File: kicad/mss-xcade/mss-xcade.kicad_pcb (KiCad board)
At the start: 2 copper layers, 82.6 x 76.2 mm, 93 parts, among them J1 Screw_Terminal_01x02, J10 Screw_Terminal_01x02, J2 SM04B-SRSS, J3 SM04B-SRSS, J4 SM04B-SRSS, J5 8P8C, J6 8P8C, J7 AVR-ISP, J8 Screw_Terminal_01x02, J9 Screw_Terminal_01x02, U1 AP7381-50Y, U2 ATtiny861A-S, U3 74HC4049, U4 AP3012

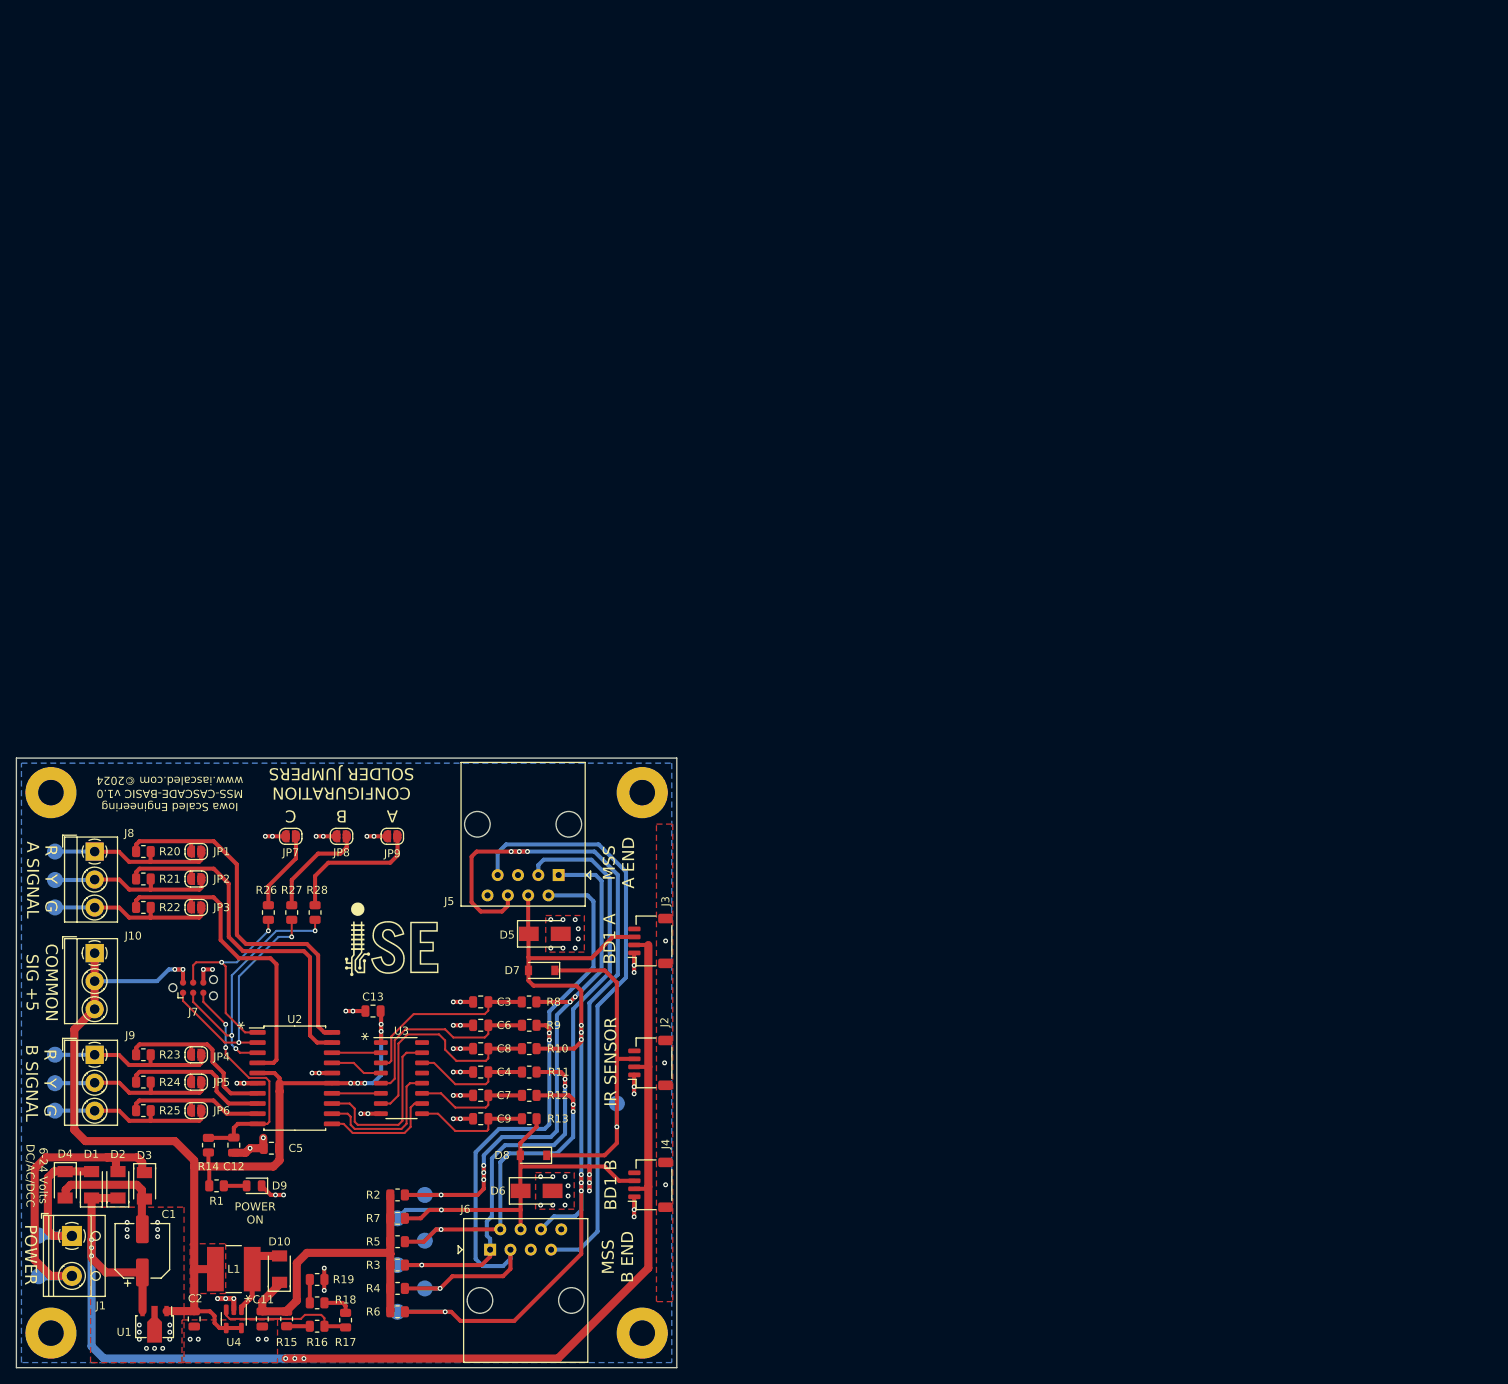
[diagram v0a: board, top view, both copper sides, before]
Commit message: First cut of xcade PCB
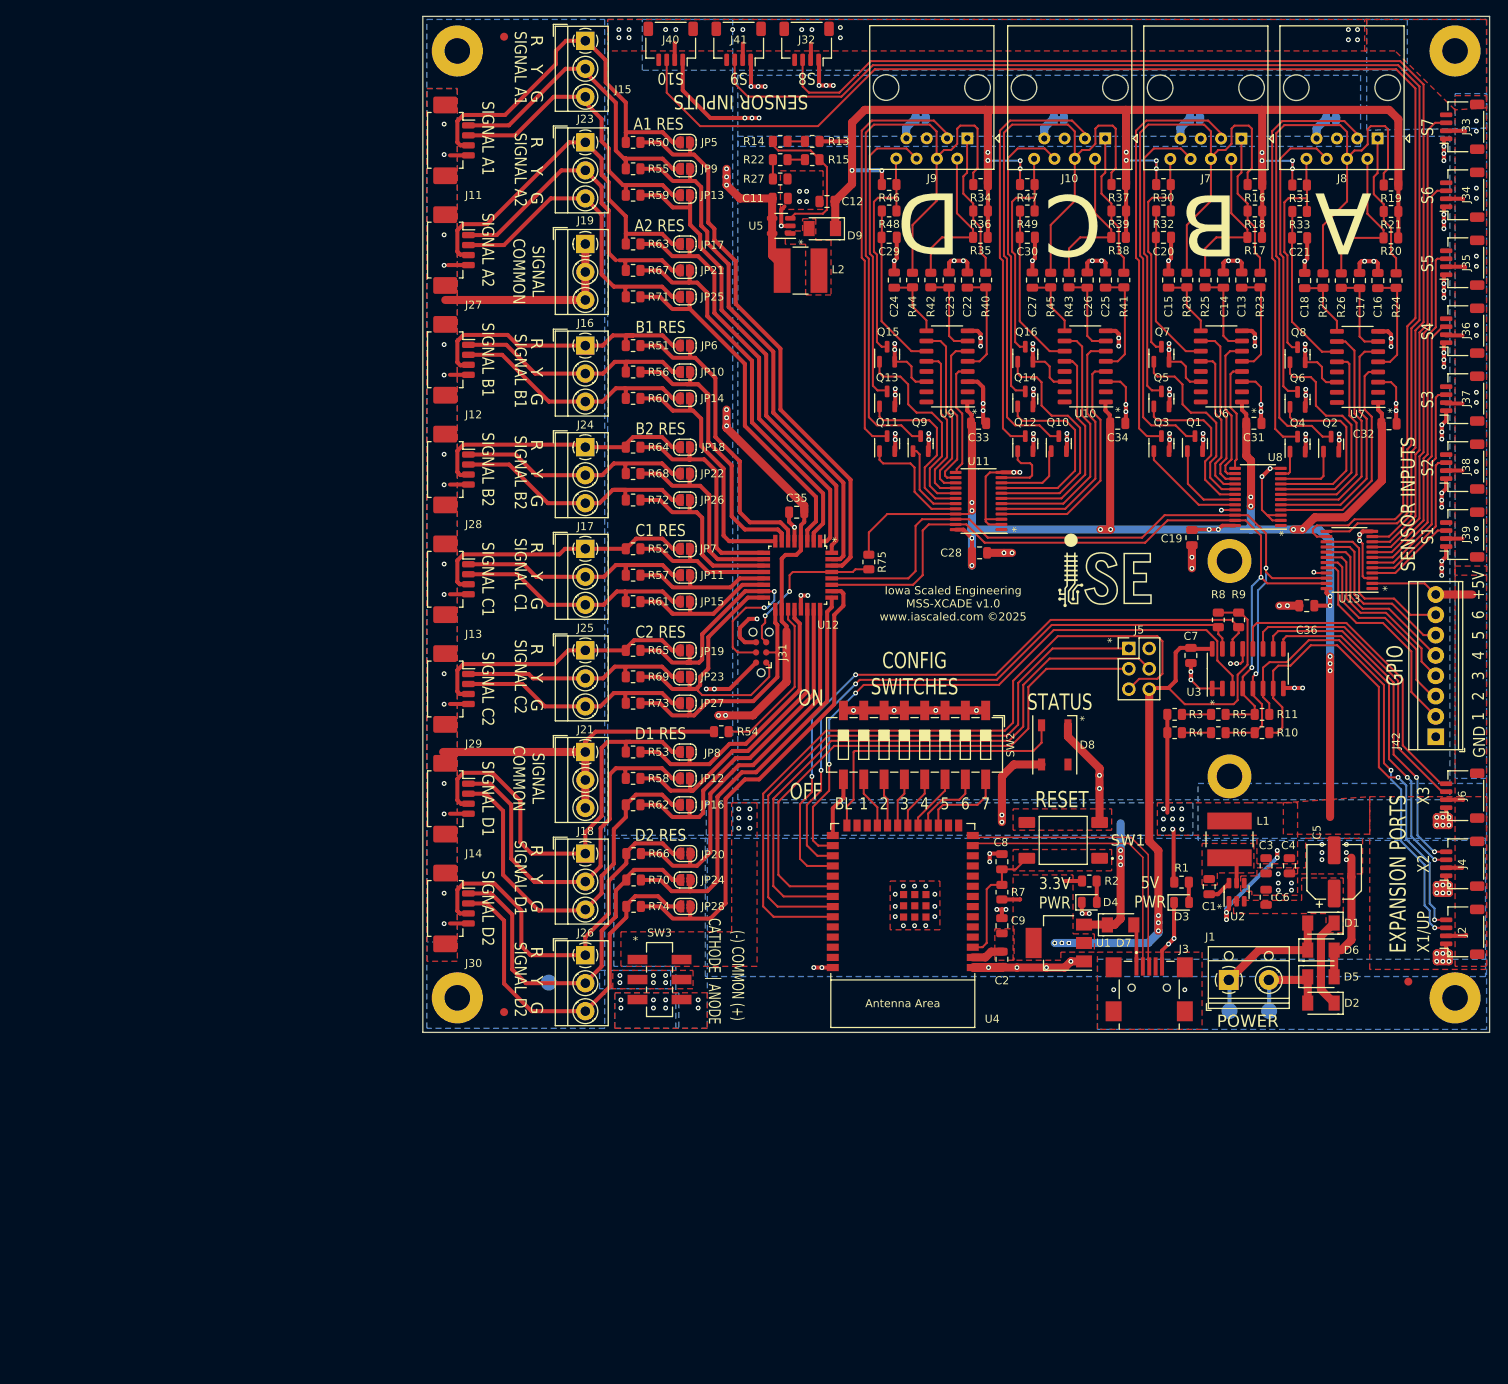
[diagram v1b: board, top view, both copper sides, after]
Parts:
- removed D10: CDBM140G, ISE_Generic:SOD-123T
- removed R12: 10k, Resistor_SMD:R_0805_2012Metric
- removed TP10, TP11, TP12, TP13, TP14, TP15, TP4, TP5, TP6, TP7, TP8, TP9: TestPoint, TestPoint:TestPoint_Pad_D2.0mm
- added C14: 0.1uF, Capacitor_SMD:C_0805_2012Metric, F.Cu at (176.3, 55.8)
- added C15: 0.1uF, Capacitor_SMD:C_0805_2012Metric, F.Cu at (169.4, 55.8)
- added C16: 0.1uF, Capacitor_SMD:C_0805_2012Metric, F.Cu at (195.6, 55.9)
- added C17: 0.1uF, Capacitor_SMD:C_0805_2012Metric, F.Cu at (193.3, 55.9)
- added C18: 0.1uF, Capacitor_SMD:C_0805_2012Metric, F.Cu at (186.4, 55.9)
- added C19: 0.1uF, Capacitor_SMD:C_0805_2012Metric, F.Cu at (172.3, 88.0)
- added C20: 0.1uF, Capacitor_SMD:C_0805_2012Metric, F.Cu at (168.8, 50.5)
- added C21: 0.1uF, Capacitor_SMD:C_0805_2012Metric, F.Cu at (185.8, 50.5)
- added C22: 0.1uF, Capacitor_SMD:C_0805_2012Metric, F.Cu at (144.3, 55.8)
- added C23: 0.1uF, Capacitor_SMD:C_0805_2012Metric, F.Cu at (142.0, 55.8)
- added C24: 0.1uF, Capacitor_SMD:C_0805_2012Metric, F.Cu at (135.1, 55.8)
- added C25: 0.1uF, Capacitor_SMD:C_0805_2012Metric, F.Cu at (161.5, 55.8)
- added C26: 0.1uF, Capacitor_SMD:C_0805_2012Metric, F.Cu at (159.3, 55.8)
- added C27: 0.1uF, Capacitor_SMD:C_0805_2012Metric, F.Cu at (152.4, 55.8)
- added C28: 0.1uF, Capacitor_SMD:C_0805_2012Metric, F.Cu at (145.8, 89.9)
- added C29: 0.1uF, Capacitor_SMD:C_0805_2012Metric, F.Cu at (134.5, 50.5)
- added C30: 0.1uF, Capacitor_SMD:C_0805_2012Metric, F.Cu at (151.8, 50.5)
- added C31: 0.1uF, Capacitor_SMD:C_0805_2012Metric, F.Cu at (180.1, 73.7)
- added C32: 0.1uF, Capacitor_SMD:C_0805_2012Metric, F.Cu at (197.0, 73.8)
- added C33: 0.1uF, Capacitor_SMD:C_0805_2012Metric, F.Cu at (145.7, 73.7)
- added C34: 0.1uF, Capacitor_SMD:C_0805_2012Metric, F.Cu at (163.1, 73.7)
- added C35: 1uF, Capacitor_SMD:C_0805_2012Metric, F.Cu at (122.9, 84.8)
- added C36: 0.1uF, Capacitor_SMD:C_0805_2012Metric, F.Cu at (186.7, 96.5)
- added H5: MountingHole, MountingHole:MountingHole_3.2mm_M3_ISO14580_Pad, F.Cu at (177.0, 117.9)
- added H6: MountingHole, MountingHole:MountingHole_3.2mm_M3_ISO14580_Pad, F.Cu at (177.0, 90.9)
- added J11: Molex 0532610471, Connector_Molex:Molex_PicoBlade_53261-0471_1x04-1MP_P1.25mm_Horizontal, F.Cu at (79.5, 38.4)
- added J12: Molex 0532610471, Connector_Molex:Molex_PicoBlade_53261-0471_1x04-1MP_P1.25mm_Horizontal, F.Cu at (79.5, 65.8)
- added J13: Molex 0532610471, Connector_Molex:Molex_PicoBlade_53261-0471_1x04-1MP_P1.25mm_Horizontal, F.Cu at (79.5, 93.2)
- added J14: Molex 0532610471, Connector_Molex:Molex_PicoBlade_53261-0471_1x04-1MP_P1.25mm_Horizontal, F.Cu at (79.5, 120.7)
- added J15: Screw_Terminal_01x02, TerminalBlock_MetzConnect:TerminalBlock_MetzConnect_Type059_RT06303HBWC_1x03_P3.50mm_Horizontal, F.Cu at (96.5, 25.9)
- added J16: Screw_Terminal_01x02, TerminalBlock_MetzConnect:TerminalBlock_MetzConnect_Type059_RT06303HBWC_1x03_P3.50mm_Horizontal, F.Cu at (96.5, 64.0)
- added J17: Screw_Terminal_01x02, TerminalBlock_MetzConnect:TerminalBlock_MetzConnect_Type059_RT06303HBWC_1x03_P3.50mm_Horizontal, F.Cu at (96.5, 89.4)
- added J18: Screw_Terminal_01x02, TerminalBlock_MetzConnect:TerminalBlock_MetzConnect_Type059_RT06303HBWC_1x03_P3.50mm_Horizontal, F.Cu at (96.5, 127.5)
- added J19: Screw_Terminal_01x02, TerminalBlock_MetzConnect:TerminalBlock_MetzConnect_Type059_RT06303HBWC_1x03_P3.50mm_Horizontal, F.Cu at (96.5, 51.3)
- added J21: Screw_Terminal_01x02, TerminalBlock_MetzConnect:TerminalBlock_MetzConnect_Type059_RT06303HBWC_1x03_P3.50mm_Horizontal, F.Cu at (96.5, 114.8)
- added J23: Screw_Terminal_01x02, TerminalBlock_MetzConnect:TerminalBlock_MetzConnect_Type059_RT06303HBWC_1x03_P3.50mm_Horizontal, F.Cu at (96.5, 38.6)
- added J24: Screw_Terminal_01x02, TerminalBlock_MetzConnect:TerminalBlock_MetzConnect_Type059_RT06303HBWC_1x03_P3.50mm_Horizontal, F.Cu at (96.5, 76.7)
- added J25: Screw_Terminal_01x02, TerminalBlock_MetzConnect:TerminalBlock_MetzConnect_Type059_RT06303HBWC_1x03_P3.50mm_Horizontal, F.Cu at (96.5, 102.1)
- added J26: Screw_Terminal_01x02, TerminalBlock_MetzConnect:TerminalBlock_MetzConnect_Type059_RT06303HBWC_1x03_P3.50mm_Horizontal, F.Cu at (96.5, 140.2)
- added J27: Molex 0532610471, Connector_Molex:Molex_PicoBlade_53261-0471_1x04-1MP_P1.25mm_Horizontal, F.Cu at (79.5, 52.1)
- added J28: Molex 0532610471, Connector_Molex:Molex_PicoBlade_53261-0471_1x04-1MP_P1.25mm_Horizontal, F.Cu at (79.5, 79.5)
- added J29: Molex 0532610471, Connector_Molex:Molex_PicoBlade_53261-0471_1x04-1MP_P1.25mm_Horizontal, F.Cu at (79.5, 106.9)
- added J30: Molex 0532610471, Connector_Molex:Molex_PicoBlade_53261-0471_1x04-1MP_P1.25mm_Horizontal, F.Cu at (79.5, 134.4)
- added J31: AVR-ISP, Connector:Tag-Connect_TC2030-IDC-NL_2x03_P1.27mm_Vertical, F.Cu at (118.5, 102.4)
- added J32: SM04B-SRSS, Connector_JST:JST_SH_SM04B-SRSS-TB_1x04-1MP_P1.00mm_Horizontal, F.Cu at (124.2, 26.3)
- added J33: SM04B-SRSS, Connector_JST:JST_SH_SM04B-SRSS-TB_1x04-1MP_P1.00mm_Horizontal, F.Cu at (206.1, 36.7)
- added J34: SM04B-SRSS, Connector_JST:JST_SH_SM04B-SRSS-TB_1x04-1MP_P1.00mm_Horizontal, F.Cu at (206.1, 45.2)
- added J35: SM04B-SRSS, Connector_JST:JST_SH_SM04B-SRSS-TB_1x04-1MP_P1.00mm_Horizontal, F.Cu at (206.1, 53.7)
- added J36: SM04B-SRSS, Connector_JST:JST_SH_SM04B-SRSS-TB_1x04-1MP_P1.00mm_Horizontal, F.Cu at (206.1, 62.1)
- added J37: SM04B-SRSS, Connector_JST:JST_SH_SM04B-SRSS-TB_1x04-1MP_P1.00mm_Horizontal, F.Cu at (206.1, 70.6)
- added J38: SM04B-SRSS, Connector_JST:JST_SH_SM04B-SRSS-TB_1x04-1MP_P1.00mm_Horizontal, F.Cu at (206.1, 79.1)
- added J39: SM04B-SRSS, Connector_JST:JST_SH_SM04B-SRSS-TB_1x04-1MP_P1.00mm_Horizontal, F.Cu at (206.1, 87.6)
- added J40: SM04B-SRSS, Connector_JST:JST_SH_SM04B-SRSS-TB_1x04-1MP_P1.00mm_Horizontal, F.Cu at (107.2, 26.3)
- added J41: SM04B-SRSS, Connector_JST:JST_SH_SM04B-SRSS-TB_1x04-1MP_P1.00mm_Horizontal, F.Cu at (115.7, 26.3)
- added J42: Screw_Terminal_01x08, TerminalBlock_TE-Connectivity:TerminalBlock_TE_282834-8_1x08_P2.54mm_Horizontal, F.Cu at (202.8, 112.9)
- added JP10: SolderJumper_2_Open, Jumper:SolderJumper-2_P1.3mm_Open_RoundedPad1.0x1.5mm, F.Cu at (109.0, 67.3)
- added JP11: SolderJumper_2_Open, Jumper:SolderJumper-2_P1.3mm_Open_RoundedPad1.0x1.5mm, F.Cu at (109.0, 92.7)
- added JP12: SolderJumper_2_Open, Jumper:SolderJumper-2_P1.3mm_Open_RoundedPad1.0x1.5mm, F.Cu at (109.0, 118.1)
- added JP13: SolderJumper_2_Open, Jumper:SolderJumper-2_P1.3mm_Open_RoundedPad1.0x1.5mm, F.Cu at (109.0, 45.2)
- added JP14: SolderJumper_2_Open, Jumper:SolderJumper-2_P1.3mm_Open_RoundedPad1.0x1.5mm, F.Cu at (109.0, 70.6)
- added JP15: SolderJumper_2_Open, Jumper:SolderJumper-2_P1.3mm_Open_RoundedPad1.0x1.5mm, F.Cu at (109.0, 96.0)
- added JP16: SolderJumper_2_Open, Jumper:SolderJumper-2_P1.3mm_Open_RoundedPad1.0x1.5mm, F.Cu at (109.0, 121.4)
- added JP17: SolderJumper_2_Open, Jumper:SolderJumper-2_P1.3mm_Open_RoundedPad1.0x1.5mm, F.Cu at (109.0, 51.3)
- added JP18: SolderJumper_2_Open, Jumper:SolderJumper-2_P1.3mm_Open_RoundedPad1.0x1.5mm, F.Cu at (109.0, 76.7)
- added JP19: SolderJumper_2_Open, Jumper:SolderJumper-2_P1.3mm_Open_RoundedPad1.0x1.5mm, F.Cu at (109.0, 102.1)
- added JP20: SolderJumper_2_Open, Jumper:SolderJumper-2_P1.3mm_Open_RoundedPad1.0x1.5mm, F.Cu at (109.0, 127.5)
- added JP21: SolderJumper_2_Open, Jumper:SolderJumper-2_P1.3mm_Open_RoundedPad1.0x1.5mm, F.Cu at (109.0, 54.6)
- added JP22: SolderJumper_2_Open, Jumper:SolderJumper-2_P1.3mm_Open_RoundedPad1.0x1.5mm, F.Cu at (109.0, 80.0)
- added JP23: SolderJumper_2_Open, Jumper:SolderJumper-2_P1.3mm_Open_RoundedPad1.0x1.5mm, F.Cu at (109.0, 105.4)
- added JP24: SolderJumper_2_Open, Jumper:SolderJumper-2_P1.3mm_Open_RoundedPad1.0x1.5mm, F.Cu at (109.0, 130.8)
- added JP25: SolderJumper_2_Open, Jumper:SolderJumper-2_P1.3mm_Open_RoundedPad1.0x1.5mm, F.Cu at (109.0, 57.9)
- added JP26: SolderJumper_2_Open, Jumper:SolderJumper-2_P1.3mm_Open_RoundedPad1.0x1.5mm, F.Cu at (109.0, 83.3)
- added JP27: SolderJumper_2_Open, Jumper:SolderJumper-2_P1.3mm_Open_RoundedPad1.0x1.5mm, F.Cu at (109.0, 108.7)
- added JP28: SolderJumper_2_Open, Jumper:SolderJumper-2_P1.3mm_Open_RoundedPad1.0x1.5mm, F.Cu at (109.0, 134.1)
- added L2: 4.7uH, ISE_UltraLibrarian:MSS6132-xxxMLC, F.Cu at (123.4, 54.6)
- added Q1: ZXMS6004FF, Package_TO_SOT_SMD:SOT-23, F.Cu at (172.7, 76.3)
- added Q10: ZXMS6004FF, Package_TO_SOT_SMD:SOT-23, F.Cu at (155.7, 76.3)
- added Q11: ZXMS6004FF, Package_TO_SOT_SMD:SOT-23, F.Cu at (134.2, 76.3)
- added Q12: ZXMS6004FF, Package_TO_SOT_SMD:SOT-23, F.Cu at (151.5, 76.3)
- added Q13: ZXMS6004FF, Package_TO_SOT_SMD:SOT-23, F.Cu at (134.2, 70.7)
- added Q14: ZXMS6004FF, Package_TO_SOT_SMD:SOT-23, F.Cu at (151.5, 70.7)
- added Q15: ZXMS6004FF, Package_TO_SOT_SMD:SOT-23, F.Cu at (134.2, 65.1)
- added Q16: ZXMS6004FF, Package_TO_SOT_SMD:SOT-23, F.Cu at (151.5, 65.1)
- added Q2: ZXMS6004FF, Package_TO_SOT_SMD:SOT-23, F.Cu at (189.7, 76.3)
- added Q3: ZXMS6004FF, Package_TO_SOT_SMD:SOT-23, F.Cu at (168.5, 76.3)
- added Q4: ZXMS6004FF, Package_TO_SOT_SMD:SOT-23, F.Cu at (185.5, 76.3)
- added Q5: ZXMS6004FF, Package_TO_SOT_SMD:SOT-23, F.Cu at (168.5, 70.7)
- added Q6: ZXMS6004FF, Package_TO_SOT_SMD:SOT-23, F.Cu at (185.5, 70.7)
- added Q7: ZXMS6004FF, Package_TO_SOT_SMD:SOT-23, F.Cu at (168.5, 65.1)
- added Q8: ZXMS6004FF, Package_TO_SOT_SMD:SOT-23, F.Cu at (185.5, 65.2)
- added Q9: ZXMS6004FF, Package_TO_SOT_SMD:SOT-23, F.Cu at (138.4, 76.3)
- added R29: 10k, Resistor_SMD:R_0805_2012Metric, F.Cu at (188.7, 55.9)
- added R30: 10k, Resistor_SMD:R_0805_2012Metric, F.Cu at (168.8, 43.9)
- added R31: 10k, Resistor_SMD:R_0805_2012Metric, F.Cu at (185.8, 43.9)
- added R32: 10k, Resistor_SMD:R_0805_2012Metric, F.Cu at (168.8, 47.2)
- added R33: 10k, Resistor_SMD:R_0805_2012Metric, F.Cu at (185.8, 47.2)
- added R34: 10k, Resistor_SMD:R_0805_2012Metric, F.Cu at (145.9, 43.9)
- added R35: 10k, Resistor_SMD:R_0805_2012Metric, F.Cu at (145.9, 50.5)
- added R36: 10k, Resistor_SMD:R_0805_2012Metric, F.Cu at (145.9, 47.2)
- added R37: 10k, Resistor_SMD:R_0805_2012Metric, F.Cu at (163.2, 43.9)
- added R38: 10k, Resistor_SMD:R_0805_2012Metric, F.Cu at (163.2, 50.5)
- added R39: 10k, Resistor_SMD:R_0805_2012Metric, F.Cu at (163.2, 47.2)
- added R40: 10k, Resistor_SMD:R_0805_2012Metric, F.Cu at (146.6, 55.8)
- added R41: 10k, Resistor_SMD:R_0805_2012Metric, F.Cu at (163.8, 55.8)
- added R42: 10k, Resistor_SMD:R_0805_2012Metric, F.Cu at (139.7, 55.8)
- added R43: 10k, Resistor_SMD:R_0805_2012Metric, F.Cu at (157.0, 55.8)
- added R44: 10k, Resistor_SMD:R_0805_2012Metric, F.Cu at (137.4, 55.8)
- added R45: 10k, Resistor_SMD:R_0805_2012Metric, F.Cu at (154.7, 55.8)
- added R46: 10k, Resistor_SMD:R_0805_2012Metric, F.Cu at (134.5, 43.9)
- added R47: 10k, Resistor_SMD:R_0805_2012Metric, F.Cu at (151.8, 43.9)
- added R48: 10k, Resistor_SMD:R_0805_2012Metric, F.Cu at (134.5, 47.2)
- added R49: 10k, Resistor_SMD:R_0805_2012Metric, F.Cu at (151.8, 47.2)
- added R50: 330, Resistor_SMD:R_0805_2012Metric, F.Cu at (102.5, 38.6)
- added R51: 330, Resistor_SMD:R_0805_2012Metric, F.Cu at (102.5, 64.0)
- added R52: 330, Resistor_SMD:R_0805_2012Metric, F.Cu at (102.5, 89.4)
- added R53: 330, Resistor_SMD:R_0805_2012Metric, F.Cu at (102.5, 114.8)
- added R54: 10k, Resistor_SMD:R_0805_2012Metric, F.Cu at (113.5, 112.3)
- added R55: 330, Resistor_SMD:R_0805_2012Metric, F.Cu at (102.5, 41.9)
- added R56: 330, Resistor_SMD:R_0805_2012Metric, F.Cu at (102.5, 67.3)
- added R57: 330, Resistor_SMD:R_0805_2012Metric, F.Cu at (102.5, 92.7)
- added R58: 330, Resistor_SMD:R_0805_2012Metric, F.Cu at (102.5, 118.1)
- added R59: 330, Resistor_SMD:R_0805_2012Metric, F.Cu at (102.5, 45.2)
- added R60: 330, Resistor_SMD:R_0805_2012Metric, F.Cu at (102.5, 70.6)
- added R61: 330, Resistor_SMD:R_0805_2012Metric, F.Cu at (102.5, 96.0)
- added R62: 330, Resistor_SMD:R_0805_2012Metric, F.Cu at (102.5, 121.4)
- added R63: 330, Resistor_SMD:R_0805_2012Metric, F.Cu at (102.5, 51.3)
- added R64: 330, Resistor_SMD:R_0805_2012Metric, F.Cu at (102.5, 76.7)
- added R65: 330, Resistor_SMD:R_0805_2012Metric, F.Cu at (102.5, 102.1)
- added R66: 330, Resistor_SMD:R_0805_2012Metric, F.Cu at (102.6, 127.5)
- added R67: 330, Resistor_SMD:R_0805_2012Metric, F.Cu at (102.5, 54.6)
- added R68: 330, Resistor_SMD:R_0805_2012Metric, F.Cu at (102.5, 80.0)
- added R69: 330, Resistor_SMD:R_0805_2012Metric, F.Cu at (102.5, 105.4)
- added R70: 330, Resistor_SMD:R_0805_2012Metric, F.Cu at (102.6, 130.8)
- added R71: 330, Resistor_SMD:R_0805_2012Metric, F.Cu at (102.5, 57.9)
- added R72: 330, Resistor_SMD:R_0805_2012Metric, F.Cu at (102.5, 83.3)
- added R73: 330, Resistor_SMD:R_0805_2012Metric, F.Cu at (102.5, 108.7)
- added R74: 330, Resistor_SMD:R_0805_2012Metric, F.Cu at (102.6, 134.1)
- added R75: 10k, Resistor_SMD:R_0805_2012Metric, F.Cu at (132.0, 91.1)
- added REF1: Fiducial_1mm_Mask2mm, Fiducial:Fiducial_1mm_Mask2mm, F.Cu at (199.4, 143.5)
- added REF2: Fiducial_1mm_Mask2mm, Fiducial:Fiducial_1mm_Mask2mm, F.Cu at (86.4, 147.3)
- added REF3: Fiducial_1mm_Mask2mm, Fiducial:Fiducial_1mm_Mask2mm, F.Cu at (86.4, 25.4)
- added SW1: FSM4JSMATR, ISE_Generic:TE_FSM4JSMA, F.Cu at (156.3, 125.9)
- added SW2: SW_DIP_x08, Button_Switch_SMD:SW_DIP_SPSTx08_Slide_6.7x21.88mm_W8.61mm_P2.54mm_LowProfile, F.Cu at (137.7, 113.9)
- added SW3: JS202011SCQN, ISE_UltraLibrarian:SW_JS202011SCQN, F.Cu at (105.8, 143.3)
- added U10: 74HC4049, Package_SO:SO-16_3.9x9.9mm_P1.27mm, F.Cu at (159.0, 66.6)
- added U11: TCA9555PWR, Package_SO:TSSOP-24_4.4x7.8mm_P0.65mm, F.Cu at (145.7, 83.4)
- added U12: ATtiny88-A, Package_QFP:TQFP-32_7x7mm_P0.8mm, F.Cu at (123.1, 92.7)
- added U13: TCA9555PWR, Package_SO:TSSOP-24_4.4x7.8mm_P0.65mm, F.Cu at (192.0, 90.8)
- added U5: AP3012, Package_TO_SOT_SMD:SOT-23-5, F.Cu at (121.0, 49.0)
- added U6: 74HC4049, Package_SO:SO-16_3.9x9.9mm_P1.27mm, F.Cu at (176.0, 66.6)
- added U7: 74HC4049, Package_SO:SO-16_3.9x9.9mm_P1.27mm, F.Cu at (193.0, 66.7)
- added U8: TCA9555PWR, Package_SO:TSSOP-24_4.4x7.8mm_P0.65mm, F.Cu at (180.6, 82.9)
- added U9: 74HC4049, Package_SO:SO-16_3.9x9.9mm_P1.27mm, F.Cu at (141.7, 66.6)
- C1: value 68uF -> 0.1uF; footprint Capacitor_SMD:CP_Elec_6.3x5.8 -> Capacitor_SMD:C_0805_2012Metric
- C11: value 10uF -> 22uF
- C12: value 1uF -> 10uF
- C3, C4: value 0.1uF -> 22uF
- C5: value 0.1uF -> 68uF; footprint Capacitor_SMD:C_0805_2012Metric -> Capacitor_SMD:CP_Elec_6.3x5.8
- C6: value 0.1uF -> 10uF
- C8: value 0.1uF -> 1uF
- D3, D4: value CDBM140G -> GREEN LED; footprint ISE_Generic:SOD-123T -> LED_SMD:LED_0805_2012Metric
- D5, D6: value SMAJ18A-TP -> CDBM140G; footprint Diode_SMD:D_SMA -> ISE_Generic:SOD-123T
- D7: footprint Diode_SMD:D_SOD-123 -> ISE_Generic:SOD-123T
- D8: value CDBM140G -> WS2812B; footprint Diode_SMD:D_SOD-123 -> LED_SMD:LED_WS2812B_PLCC4_5.0x5.0mm_P3.2mm
- D9: value GREEN LED -> CDBM140G; footprint LED_SMD:LED_0805_2012Metric -> ISE_Generic:SOD-123T
- J10, J8, J9: value Screw_Terminal_01x02 -> 8P8C; footprint TerminalBlock_MetzConnect:TerminalBlock_MetzConnect_Type059_RT06303HBWC_1x03_P3.50mm_Horizontal -> Connector_RJ:RJ45_Amphenol_54602-x08_Horizontal
- J3: value SM04B-SRSS -> 690-005-299-043; footprint Connector_JST:JST_SH_SM04B-SRSS-TB_1x04-1MP_P1.00mm_Horizontal -> ISE_UltraLibrarian:EDAC_690-005-299-043
- J5: value 8P8C -> Conn_02x03_Odd_Even; footprint Connector_RJ:RJ45_Amphenol_54602-x08_Horizontal -> Connector_PinHeader_2.54mm:PinHeader_2x03_P2.54mm_Vertical
- J6: value 8P8C -> SM04B-SRSS; footprint Connector_RJ:RJ45_Amphenol_54602-x08_Horizontal -> Connector_JST:JST_SH_SM04B-SRSS-TB_1x04-1MP_P1.00mm_Horizontal
- J7: value AVR-ISP -> 8P8C; footprint Connector:Tag-Connect_TC2030-IDC-NL_2x03_P1.27mm_Vertical -> Connector_RJ:RJ45_Amphenol_54602-x08_Horizontal
- JP1, JP2, JP3, JP4: value SolderJumper_2_Open -> SolderJumper_2_Bridged; footprint Jumper:SolderJumper-2_P1.3mm_Open_RoundedPad1.0x1.5mm -> Jumper:SolderJumper-2_P1.3mm_Bridged_RoundedPad1.0x1.5mm; moved to B.Cu
- R10, R11: value 10k -> 0
- R15, R2, R3, R4, R5, R6: value 10k -> 1k
- R17, R18, R26, R28: value 1k -> 10k
- R19, R20, R21, R23, R24, R25: value 330 -> 10k
- R22: value 330 -> 1k
- R27: value 1k -> 330
- U1: value AP7381-50Y -> AZ1117-3.3; footprint ISE_Generic:SOT-89-3 -> Package_TO_SOT_SMD:SOT-223-3_TabPin2
- U2: value ATtiny861A-S -> AP63205WU; footprint Package_SO:SOIC-20W_7.5x12.8mm_P1.27mm -> Package_TO_SOT_SMD:TSOT-23-6
- U3: value 74HC4049 -> PCA9546ADR; footprint Package_SO:SO-16_3.9x9.9mm_P1.27mm -> Package_SO:SOIC-16_3.9x9.9mm_P1.27mm
- U4: value AP3012 -> ESP32-S2-SOLO; footprint Package_TO_SOT_SMD:SOT-23-5 -> ISE_Generic:ESP32-S2-SOLO
- moved R19 191.7 mm to (197.2, 43.9), turned to 0 degrees
- moved R24 185.9 mm to (197.9, 55.9), turned to -90 degrees
- moved R16 184.7 mm to (180.2, 43.9), turned to 0 degrees
- moved J8 183.5 mm to (195.5, 38.1), turned to 180 degrees
- moved H1 180.4 mm to (205.2, 145.5)
- moved R18 179.9 mm to (180.2, 47.2)
- moved R21 176.9 mm to (197.2, 47.2)
- moved R17 176.7 mm to (180.2, 50.5), turned to 0 degrees
- moved R20 173.8 mm to (197.2, 50.5)
- moved JP2 170.7 mm to (189.7, 35.7), turned to 180 degrees
- moved R23 169.9 mm to (180.8, 55.8), turned to -90 degrees
- moved J7 168.6 mm to (178.5, 38.1), turned to 180 degrees
- moved R25 168.5 mm to (174.0, 55.8), turned to -90 degrees
- moved J10 162.3 mm to (161.5, 38.1), turned to 180 degrees
- moved H2 161.9 mm to (80.5, 27.2)
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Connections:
- C1 pad 1: /VPWR -> Net-(C1-Pad1)
- C1 pad 2: GND -> Net-(C1-Pad2)
- C11 pad 1: +12V -> +5V
- C12 pad 1: Net-(C12-Pad1) -> +12V
- C13 pad 1: +5V -> Net-(C13-Pad1)
- C2 pad 1: +5V -> +3.3V
- C3 pad 1: Net-(C3-Pad1) -> +5V
- C4 pad 1: Net-(C4-Pad1) -> +5V
- C5 pad 1: +5V -> /VPWR
- C6 pad 1: Net-(C6-Pad1) -> /VPWR
- C7 pad 1: Net-(C7-Pad1) -> +3.3V
- C8 pad 1: Net-(C8-Pad1) -> /~{RST}
- C9 pad 1: Net-(C9-Pad1) -> +3.3V
- D3 pad 1: Net-(D2-Pad2) -> GND
- D3 pad 2: GND -> Net-(D3-Pad2)
- D4 pad 1: Net-(D1-Pad2) -> GND
- D4 pad 2: GND -> Net-(D4-Pad2)
- D5 pad 1: /A_ADJACENT -> Net-(D2-Pad2)
- D6 pad 1: /B_ADJACENT -> Net-(D1-Pad2)
- D7 pad 1: Net-(D7-Pad1) -> +5V
- D7 pad 2: /A_ADJACENT -> Net-(D7-Pad2)
- D8 pad 1: Net-(D7-Pad1) -> +5V
- D8 pad 2: /B_ADJACENT -> unconnected-(D8-Pad2)
- D9 pad 1: GND -> +12V
- J10 pad 1: +5V -> Net-(J10-Pad1)
- J10 pad 2: +5V -> Net-(J10-Pad2)
- J10 pad 3: +5V -> Net-(J10-Pad3)
- J2 pad 2: /VPWR -> +5V
- J2 pad 3: Net-(D7-Pad1) -> Net-(J2-Pad3)
- J2 pad 4: unconnected-(J2-Pad4) -> Net-(J2-Pad4)
- J2 pad MP: GND -> +5V
- J3 pad 1: GND -> Net-(D7-Pad2)
- J3 pad 2: /VPWR -> /D-
- J3 pad 3: /A_ADJACENT -> /D+
- J4 pad 2: /VPWR -> +5V
- J4 pad 3: /B_ADJACENT -> Net-(J4-Pad3)
- J4 pad 4: unconnected-(J4-Pad4) -> Net-(J4-Pad4)
- J4 pad MP: GND -> +5V
- J5 pad 1: Net-(J5-Pad1) -> /CAN_AUX1
- J5 pad 2: Net-(J5-Pad2) -> GND
- J5 pad 3: Net-(J5-Pad3) -> /CAN_TX
- J5 pad 4: /A_ADJACENT -> /CAN_RX
- J5 pad 5: GND -> /CAN_AUX2
- J5 pad 6: /B_ADJACENT -> +3.3V
- J6 pad 1: Net-(J6-Pad1) -> GND
- J6 pad 2: Net-(J5-Pad3) -> +5V
- J6 pad 3: Net-(J5-Pad2) -> Net-(J6-Pad3)
- J6 pad 4: /B_ADJACENT -> Net-(J6-Pad4)
- J7 pad 2: +5V -> Net-(J7-Pad2)
- J7 pad 5: Net-(C12-Pad1) -> GND
- J7 pad 6: GND -> Net-(J7-Pad6)
- JP1 pad 1: /A_SIGNAL_R -> GND
- JP1 pad 2: Net-(J8-Pad1) -> Net-(J7-Pad7)
- JP2 pad 1: /A_SIGNAL_Y -> GND
- JP2 pad 2: Net-(J8-Pad2) -> Net-(J8-Pad7)
- JP3 pad 1: /A_SIGNAL_G -> GND
- JP3 pad 2: Net-(J8-Pad3) -> Net-(J9-Pad7)
- JP4 pad 1: /B_SIGNAL_R -> GND
- JP4 pad 2: Net-(J9-Pad1) -> Net-(J10-Pad7)
- JP5 pad 1: /B_SIGNAL_Y -> /Signals & Sensors/A1_SIGNAL_R
- JP5 pad 2: Net-(J9-Pad2) -> Net-(J11-Pad3)
- JP6 pad 1: /B_SIGNAL_G -> /Signals & Sensors/B1_SIGNAL_R
- JP6 pad 2: Net-(J9-Pad3) -> Net-(J12-Pad3)
- JP7 pad 1: Net-(JP7-Pad1) -> /Signals & Sensors/C1_SIGNAL_R
- JP7 pad 2: GND -> Net-(J13-Pad3)
- JP8 pad 1: Net-(JP8-Pad1) -> /Signals & Sensors/D1_SIGNAL_R
- JP8 pad 2: GND -> Net-(J14-Pad3)
- JP9 pad 1: Net-(JP9-Pad1) -> /Signals & Sensors/A1_SIGNAL_Y
- JP9 pad 2: GND -> Net-(J11-Pad1)
- L1 pad 1: +5V -> Net-(C1-Pad1)
- L1 pad 2: Net-(D10-Pad2) -> +5V
- R1 pad 1: Net-(D9-Pad2) -> Net-(D3-Pad2)
- R10 pad 1: Net-(C8-Pad1) -> Net-(J2-Pad4)
- R10 pad 2: /A_ADJACENT -> SCL
- R11 pad 1: Net-(C4-Pad1) -> Net-(J2-Pad3)
- R11 pad 2: Net-(J6-Pad1) -> SDA
- R13 pad 1: Net-(C9-Pad1) -> Net-(R13-Pad1)
- R13 pad 2: /B_ADJACENT -> +12V
- R14 pad 1: Net-(C12-Pad1) -> Net-(R14-Pad1)
- R14 pad 2: +5V -> Net-(R13-Pad1)
- R15 pad 2: +12V -> Net-(R14-Pad1)
- R16 pad 1: Net-(R16-Pad1) -> Net-(J7-Pad4)
- R16 pad 2: Net-(R15-Pad1) -> +12V
- R17 pad 1: Net-(R17-Pad1) -> Net-(J7-Pad2)
- R17 pad 2: Net-(R16-Pad1) -> +12V
- R18 pad 1: Net-(R18-Pad1) -> Net-(J7-Pad1)
- R18 pad 2: Net-(R17-Pad1) -> +12V
- R19 pad 1: GND -> Net-(J8-Pad4)
- R19 pad 2: Net-(R18-Pad1) -> +12V
- R2 pad 1: Net-(J5-Pad1) -> Net-(D4-Pad2)
- R2 pad 2: +12V -> +3.3V
- R20 pad 1: /A_SIGNAL_R -> Net-(J8-Pad2)
- R20 pad 2: Net-(J8-Pad1) -> +12V
- R21 pad 1: /A_SIGNAL_Y -> Net-(J8-Pad1)
- R21 pad 2: Net-(J8-Pad2) -> +12V
- R22 pad 1: /A_SIGNAL_G -> Net-(R22-Pad1)
- R22 pad 2: Net-(J8-Pad3) -> Net-(R15-Pad1)
- R23 pad 1: /B_SIGNAL_R -> Net-(J7-Pad1)
- R23 pad 2: Net-(J9-Pad1) -> Net-(C13-Pad1)
- R24 pad 1: /B_SIGNAL_Y -> Net-(J8-Pad1)
- R24 pad 2: Net-(J9-Pad2) -> Net-(C16-Pad1)
- R25 pad 1: /B_SIGNAL_G -> Net-(J7-Pad2)
- R25 pad 2: Net-(J9-Pad3) -> Net-(C14-Pad1)
- R26 pad 1: Net-(J7-Pad4) -> Net-(J8-Pad2)
- R26 pad 2: Net-(JP7-Pad1) -> Net-(C17-Pad1)
- R27 pad 1: Net-(J7-Pad1) -> GND
- R27 pad 2: Net-(JP8-Pad1) -> Net-(R22-Pad1)
- R28 pad 1: Net-(J7-Pad3) -> Net-(J7-Pad4)
- R28 pad 2: Net-(JP9-Pad1) -> Net-(C15-Pad1)
- R3 pad 1: Net-(J6-Pad1) -> Net-(R3-Pad1)
- R3 pad 2: +12V -> +5V
- R4 pad 1: Net-(J5-Pad2) -> Net-(R4-Pad1)
- R4 pad 2: +12V -> +5V
- R5 pad 1: Net-(J5-Pad3) -> SDA
- R5 pad 2: +12V -> Net-(R3-Pad1)
- R6 pad 1: /A_ADJACENT -> SCL
- R6 pad 2: +12V -> Net-(R4-Pad1)
- R7 pad 1: /B_ADJACENT -> /~{RST}
- R7 pad 2: +12V -> +3.3V
- R8 pad 1: Net-(C3-Pad1) -> Net-(R8-Pad1)
- R8 pad 2: Net-(J5-Pad1) -> +3.3V
- R9 pad 1: Net-(C6-Pad1) -> Net-(R9-Pad1)
- R9 pad 2: Net-(J5-Pad2) -> +3.3V
- TP1 pad 1: Net-(D7-Pad1) -> Net-(D1-Pad2)
- TP2 pad 1: Net-(J8-Pad1) -> Net-(D2-Pad2)
- TP3 pad 1: Net-(J8-Pad2) -> Net-(J11-Pad4)
- U1 pad 1: +5V -> GND
- U1 pad 2: GND -> +3.3V
- U1 pad 3: /VPWR -> +5V
- U2 pad 1: Net-(J7-Pad4) -> +5V
- U2 pad 2: Net-(J7-Pad1) -> /VPWR
- U2 pad 3: Net-(J7-Pad3) -> /VPWR
- U2 pad 4: /A_SIGNAL_G -> GND
- U2 pad 5: +5V -> Net-(C1-Pad1)
- U2 pad 6: GND -> Net-(C1-Pad2)
- U3 pad 1: +5V -> GND
- U3 pad 10: /B_ADJACENT_5V -> Net-(J4-Pad4)
- U3 pad 11: Net-(C7-Pad1) -> Net-(J6-Pad3)
- U3 pad 12: /B_APPROACH_5V -> Net-(J6-Pad4)
- U3 pad 13: (no net) -> GND
- U3 pad 14: Net-(C4-Pad1) -> Net-(R9-Pad1)
- U3 pad 15: /B_ADV_APPROACH_5V -> Net-(R8-Pad1)
- U3 pad 16: (no net) -> +3.3V
- U3 pad 2: /A_ADV_APPROACH_5V -> GND
- U3 pad 3: Net-(C3-Pad1) -> Net-(U3-Pad3)
- U3 pad 4: /A_APPROACH_5V -> SDA
- U3 pad 5: Net-(C6-Pad1) -> SCL
- U3 pad 6: /A_ADJACENT_5V -> Net-(J2-Pad3)
- U3 pad 7: Net-(C8-Pad1) -> Net-(J2-Pad4)
- U3 pad 9: Net-(C9-Pad1) -> Net-(J4-Pad3)
- U4 pad 1: Net-(D10-Pad2) -> GND
- U4 pad 2: GND -> +3.3V
- U4 pad 3: Net-(R16-Pad1) -> /~{RST}
- U4 pad 4: +5V -> unconnected-(U4-Pad4)
- U4 pad 5: +5V -> unconnected-(U4-Pad5)
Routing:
- net GND: track 74.4 -> 368.8 mm, vias 81 -> 190
- net +5V: track 140.6 -> 377.3 mm, vias 7 -> 81
- net /Signals & Sensors/SENSOR_IN_9: track 0.00 -> 171.4 mm
- net /Signals & Sensors/SENSOR_IN_8: track 0.00 -> 157.0 mm
- net /VPWR: track 158.5 -> 11.4 mm, vias 6 -> 0
- net /Signals & Sensors/SENSOR_IN_7: track 0.00 -> 144.5 mm
- net /B_ADJACENT: track 128.4 -> 0.00 mm, vias 7 -> 0
- net +12V: track 55.8 -> 182.4 mm, vias 0 -> 14
- net /A_ADJACENT: track 115.5 -> 0.00 mm, vias 7 -> 0
- net SCL: track 0.00 -> 102.2 mm, vias 0 -> 2
- net SDA: track 0.00 -> 99.0 mm, vias 0 -> 2
- net /CAN_AUX2: track 0.00 -> 93.8 mm
- net +3.3V: track 0.00 -> 93.2 mm, vias 0 -> 6
- net Net-(J5-Pad2): track 88.0 -> 0.00 mm, vias 3 -> 0
- net Net-(J9-Pad4): track 0.00 -> 87.1 mm
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- added copper zone on F.Cu, net +3.3V
- added copper zone on B.Cu, net +5V
- added copper zone on F.Cu, net /VPWR
- added copper zone on F.Cu, net /~{RST}
- added copper zone on F.Cu, net Net-(C1-Pad1)
- added copper zone on F.Cu, net Net-(D9-Pad2)
- added copper zone on B.Cu, net Net-(J11-Pad4)
- added copper zone on F.Cu, net Net-(J11-Pad4)
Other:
- board size 82.6 x 76.2 mm -> 133.4 x 127 mm
- board text added: "(-) COMMON (+)"
- board text added: "+5V"
- board text added: "1"
- board text added: "2"
- board text added: "3"
- board text added: "3.3V PWR"
- board text added: "4"
- board text added: "5"
- board text added: "5V PWR"
- board text added: "6"
- board text added: "7"
- board text added: "A1 RES"
- board text added: "A2 RES"
- board text added: "B1 RES"
- board text added: "B2 RES"
- board text added: "BL"
- board text added: "C1 RES"
- board text added: "C2 RES"
- board text added: "CATHODE | ANODE"
- board text added: "CONFIG SWITCHES"
- board text added: "D"
- board text added: "D1 RES"
- board text added: "D2 RES"
- board text added: "EXPANSION PORTS"
- board text added: "GND"
- board text added: "GPIO"
- board text added: "Iowa Scaled Engineering MSS-XCADE v1.0 www.iascaled.com ©2025"
- board text added: "OFF"
- board text added: "ON"
- board text added: "RESET"
- board text added: "S1"
- board text added: "S10"
- board text added: "S2"
- board text added: "S3"
- board text added: "S4"
- board text added: "S5"
- board text added: "S6"
- board text added: "S7"
- board text added: "S8"
- board text added: "S9"
- board text added: "SENSOR INPUTS"
- board text added: "SIGNAL A1"
- board text added: "SIGNAL A2"
- board text added: "SIGNAL B1"
- board text added: "SIGNAL B2"
- board text added: "SIGNAL C1"
- board text added: "SIGNAL C2"
- board text added: "SIGNAL COMMON"
- board text added: "SIGNAL D1"
- board text added: "SIGNAL D2"
- board text added: "STATUS"
- board text added: "X1/UP"
- board text added: "X2"
- board text added: "X3"
- board text removed: "6-24 Volts DC/AC/DCC"
- board text removed: "A SIGNAL"
- board text removed: "B SIGNAL"
- board text removed: "BD1 A"
- board text removed: "BD1 B"
- board text removed: "COMMON SIG +5"
- board text removed: "CONFIGURATION SOLDER JUMPERS"
- board text removed: "IR SENSOR"
- board text removed: "Iowa Scaled Engineering MSS-CASCADE-BASIC v1.0 www.iascaled.com ©2024"
- board text removed: "MSS A END"
- board text removed: "MSS B END"
- board text removed: "POWER ON"
